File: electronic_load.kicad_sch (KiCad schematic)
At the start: 49 parts, among them J1 Barrel_Jack_Switch_Pin3Ring, J2 Conn_01x03, J3 Conn_01x03_Pin, J4 Conn_01x06_Pin, J5 Conn_01x04_Pin, J6 Conn_02x07_Top_Bottom, J7 USB_C_Receptacle_USB2.0_16P, U1 STM32G491METx, U2 MCP4728, U3 LF33_TO252, U4 NCP1117-5.0_SOT223, U5 USBLC6-2SC6, Y1 12MHz

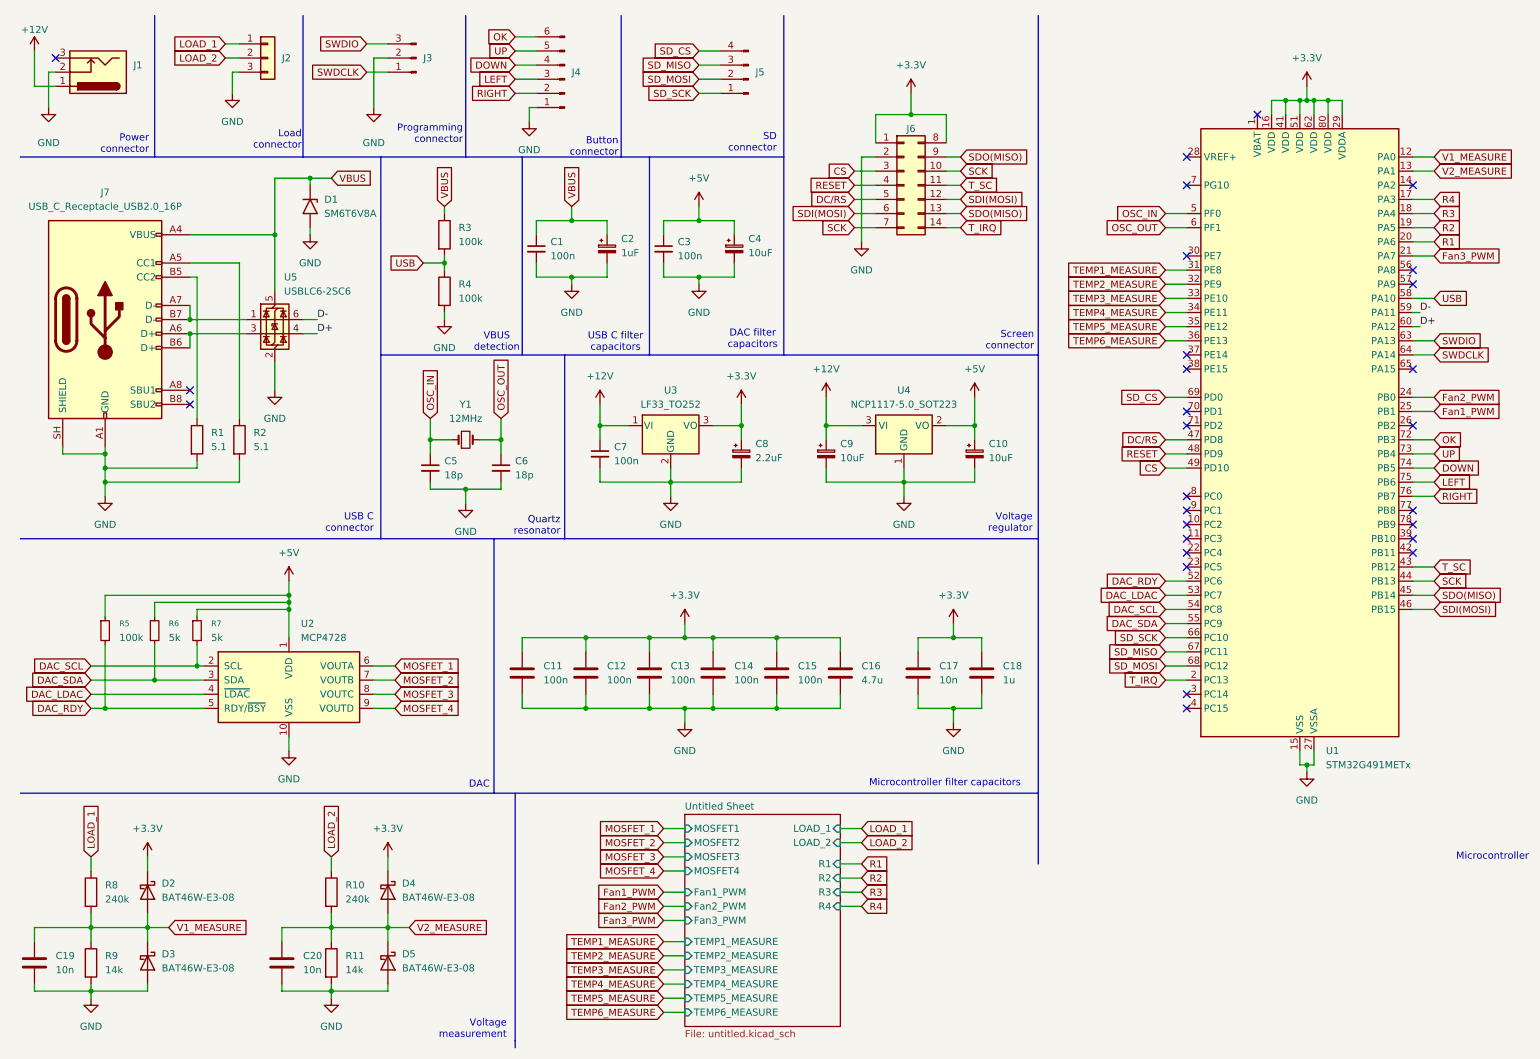
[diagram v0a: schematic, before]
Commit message: connectors
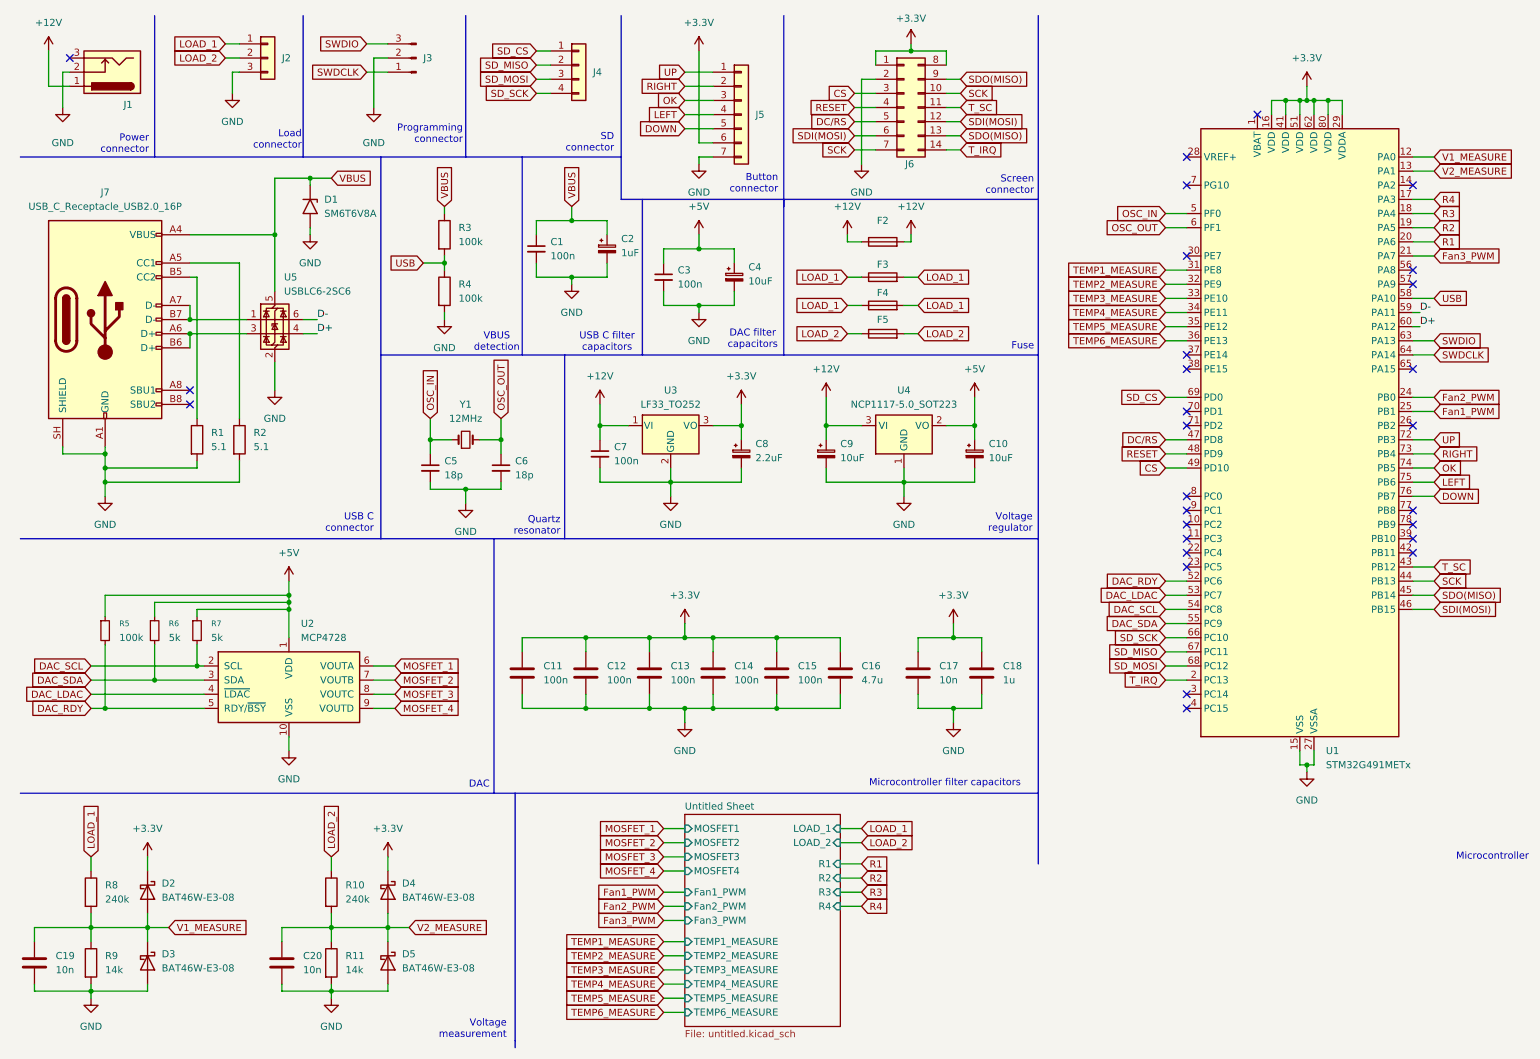
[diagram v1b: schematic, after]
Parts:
- removed J4: Conn_01x06_Pin, Connector_PinSocket_2.54mm:PinSocket_1x06_P2.54mm_Vertical, symbol Connector:Conn_01x06_Pin
- removed J5: Conn_01x04_Pin, Connector_PinSocket_2.54mm:PinSocket_1x04_P2.54mm_Vertical, symbol Connector:Conn_01x04_Pin
- added F2, F3, F4, F5: Fuse, Fuse:Fuse_1206_3216Metric_Pad1.42x1.75mm_HandSolder, symbol Device:Fuse
- added J4: Conn_01x04, Connector_JST:JST_EH_B4B-EH-A_1x04_P2.50mm_Vertical, symbol Connector_Generic:Conn_01x04
- added J5: Conn_01x07, Connector_JST:JST_EH_B7B-EH-A_1x07_P2.50mm_Vertical, symbol Connector_Generic:Conn_01x07
- J2: footprint Connector_Samtec_HPM_THT:Samtec_HPM-03-01-x-S_Straight_1x03_Pitch5.08mm -> TerminalBlock:TerminalBlock_MaiXu_MX126-5.0-03P_1x03_P5.00mm
- J3: footprint Connector_PinSocket_2.54mm:PinSocket_1x03_P2.54mm_Vertical -> Connector_PinHeader_2.54mm:PinHeader_1x03_P2.54mm_Vertical
- J6: footprint Connector_PinSocket_2.54mm:PinSocket_2x07_P2.54mm_Vertical -> Connector_JST:JST_PHD_B14B-PHDSS_2x07_P2.00mm_Vertical
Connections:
- net +12V: now also F2.1, F2.2
- net +3.3V: now also J5.6 (Pin_6)
- net DOWN: now also U1.76 (PB7), J5.5 (Pin_5); no longer U1.74 (PB5)
- net GND: now also J5.7 (Pin_7)
- net LEFT: now also J5.4 (Pin_4)
- net LOAD_1: now also F3.1, F3.2, F4.1, F4.2
- net LOAD_2: now also F5.1, F5.2
- net OK: now also U1.74 (PB5), J5.3 (Pin_3); no longer U1.72 (PB3)
- net RIGHT: now also U1.73 (PB4), J5.2 (Pin_2); no longer U1.76 (PB7)
- net SD_CS: now also J4.1 (Pin_1)
- net SD_MISO: now also J4.2 (Pin_2)
- net SD_MOSI: now also J4.3 (Pin_3)
- net SD_SCK: now also J4.4 (Pin_4)
- net UP: now also U1.72 (PB3), J5.1 (Pin_1); no longer U1.73 (PB4)
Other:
- note added: "Fuse"
- moved on the sheet: C3, C4, J1, J6

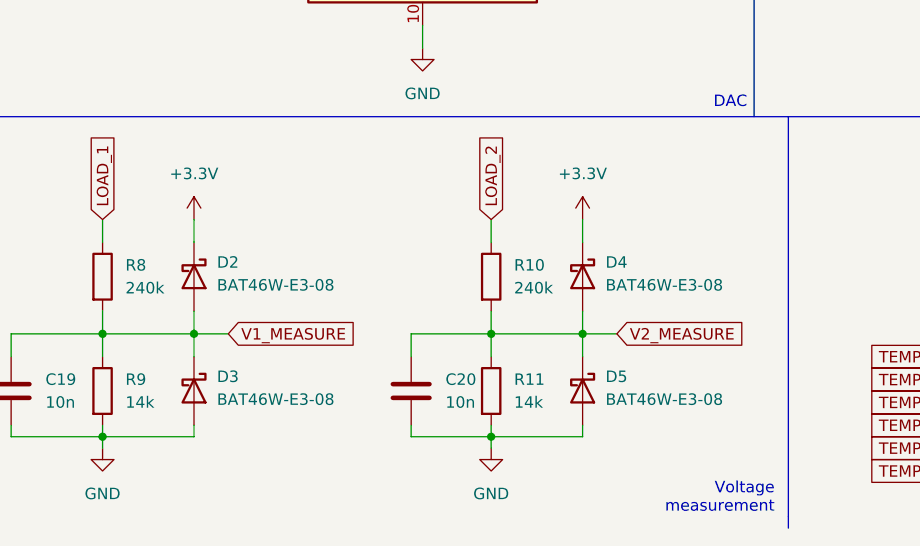
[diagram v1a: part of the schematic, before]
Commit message: zener diodes
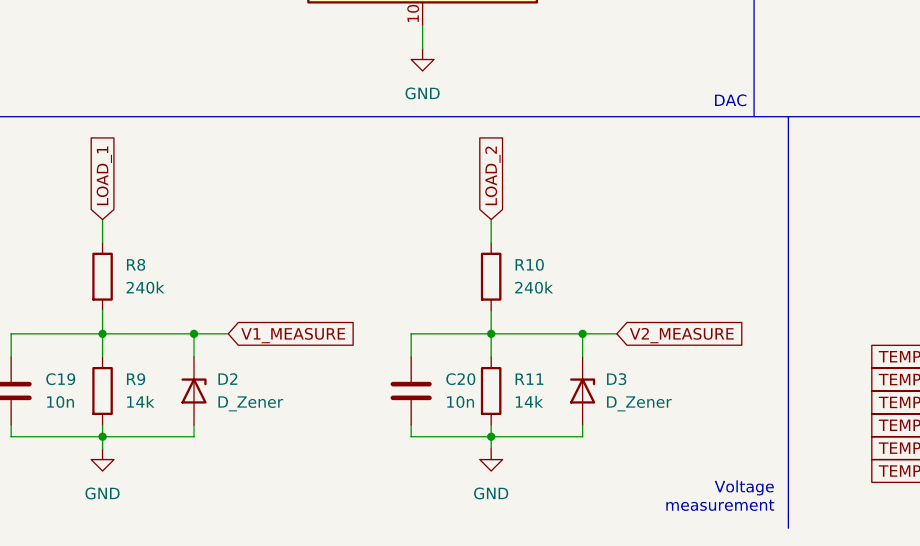
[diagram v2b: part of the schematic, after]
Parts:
- removed D2, D3, D4, D5: BAT46W-E3-08, Diode_SMD:D_SOD-123, symbol Device:D_Schottky
- added D2, D3: D_Zener, Diode_SMD:D_SOD-123F, symbol Device:D_Zener
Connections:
- net GND: now also D2.2 (A), D3.2 (A)
- net V1_MEASURE: now also D2.1 (K)
- net V2_MEASURE: now also D3.1 (K)
